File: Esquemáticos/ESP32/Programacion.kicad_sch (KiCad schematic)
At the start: 8 parts

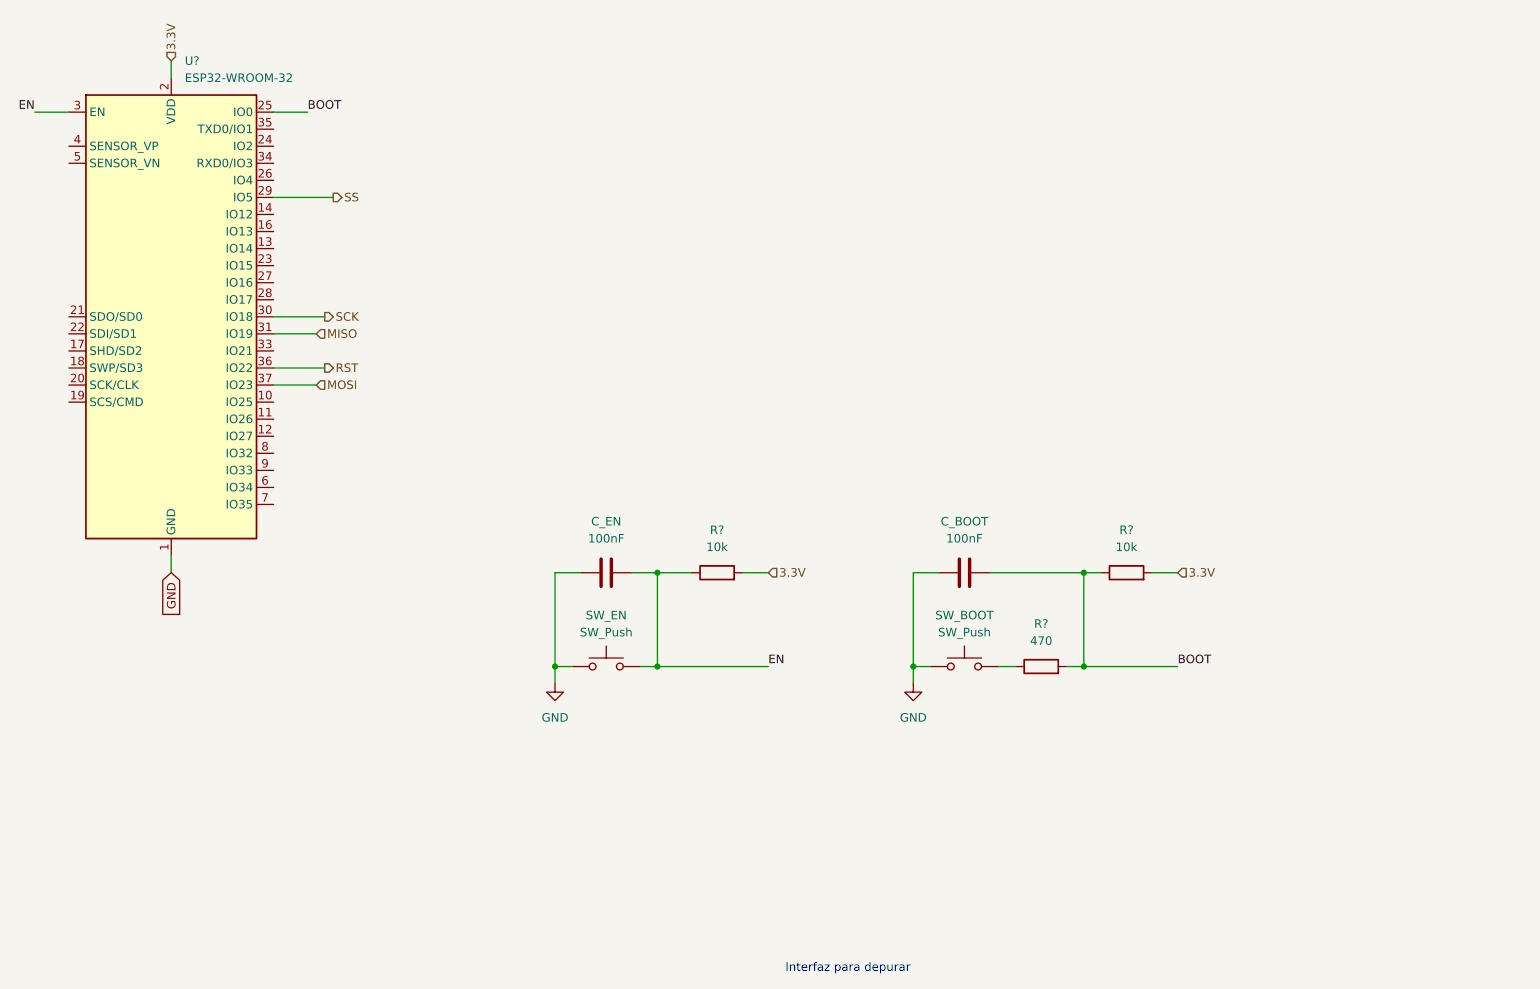
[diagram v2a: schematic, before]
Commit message: actualizacion raul 3.0
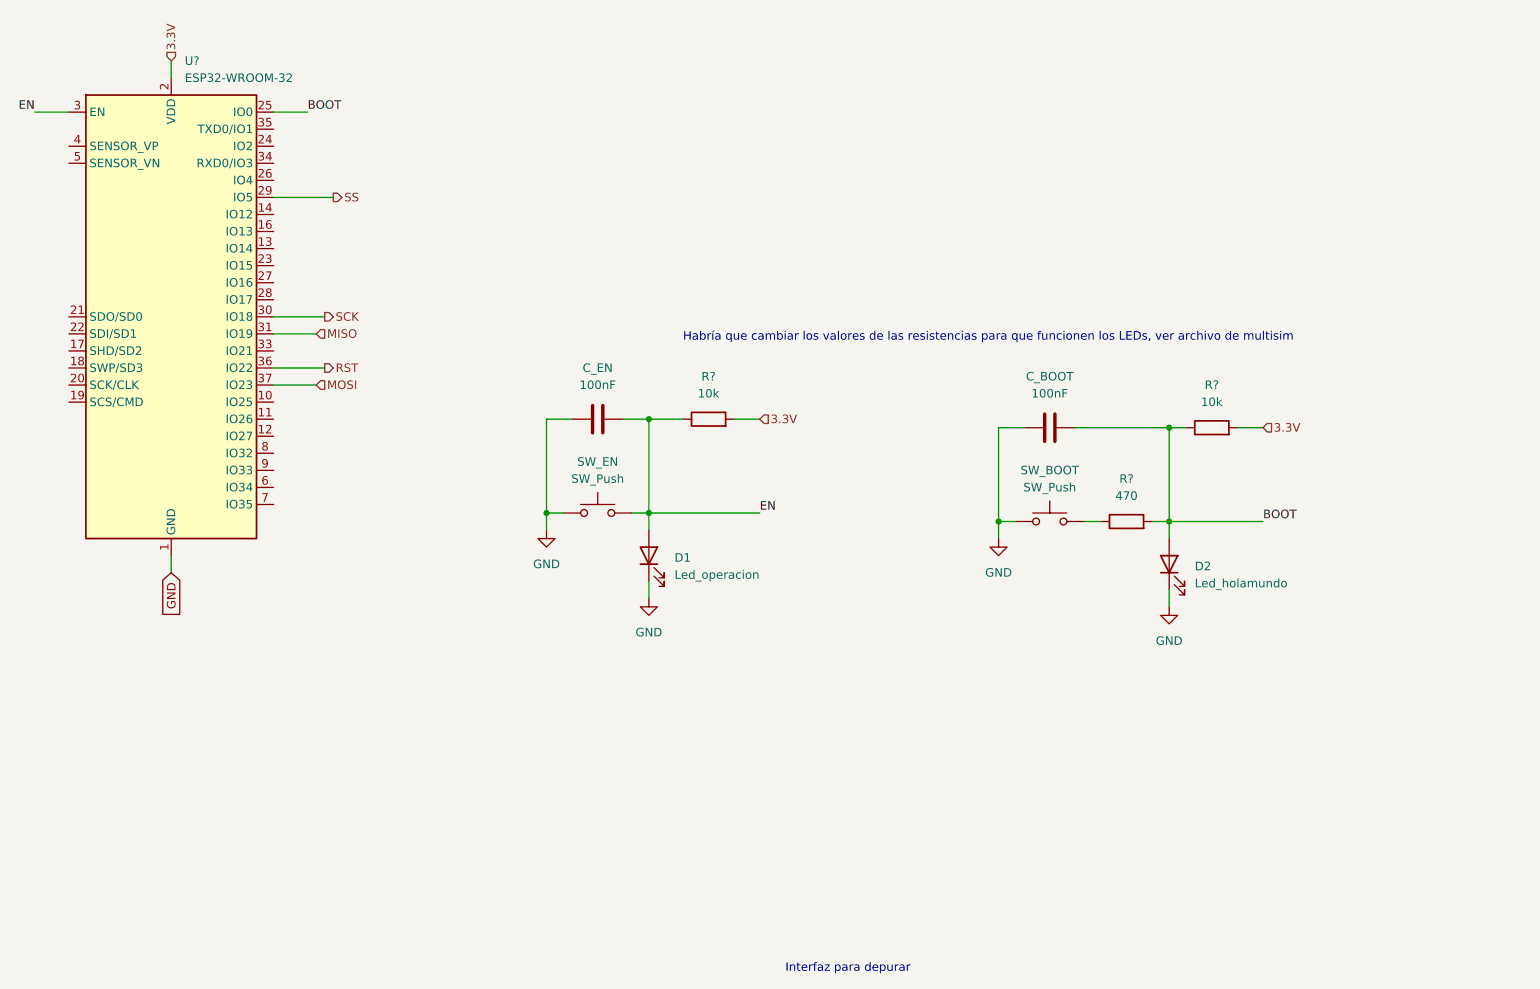
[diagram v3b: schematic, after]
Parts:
- added D1: Led_operacion, LED_SMD:LED_1206_3216Metric, symbol LED:IR26-21C_L110_TR8
- added D2: Led_holamundo, LED_SMD:LED_1206_3216Metric, symbol LED:IR26-21C_L110_TR8
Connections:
- net BOOT: now also D2.2 (A)
- net EN: now also D1.2 (A)
- net GND: now also D1.1 (K), D2.1 (K)
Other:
- note added: "Habría que cambiar los valores de las resistencias para que funcionen los LEDs, ver archivo de multisim"
- moved on the sheet: C_BOOT, C_EN, R?, SW_BOOT, SW_EN
